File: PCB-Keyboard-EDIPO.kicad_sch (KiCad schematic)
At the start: 0 parts

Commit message: MCU Edits
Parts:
- added C1: 1u, symbol Device:C_Small
- added C2, C3: 22p, symbol Device:C_Small
- added C4, C5, C6, C7: 0.1u, symbol Device:C_Small
- added C8: 10u, symbol Device:C_Small
- added J1: AVR-ISP-6, symbol Connector:AVR-ISP-6
- added R1: 10k, symbol Device:R_Small
- added U1: ATmega32U4-A, Package_QFP:TQFP-44_10x10mm_P0.8mm, symbol MCU_Microchip_ATmega:ATmega32U4-A
- added Y1: XTAL, symbol Device:Crystal_GND24_Small
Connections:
- new net: R1.1, U1.33 (~{HWB}/PE2)
- new net: C1.1, U1.6 (UCAP)
- new net +5V: C4.1, C5.1, C6.1, C7.1, C8.1, J1.2 (VCC), U1.14 (VCC), U1.2 (UVCC), U1.24 (AVCC), U1.34 (VCC), U1.44 (AVCC)
- new net D+: U1.4 (D+)
- new net D-: U1.3 (D-)
- new net GND: C1.2, C2.2, C3.2, C4.2, C5.2, C6.2, C7.2, C8.2, J1.6 (GND), R1.2, U1.15 (GND), U1.23 (GND), U1.35 (GND), U1.43 (GND), U1.5 (UGND), Y1.2, Y1.4
- new net MISO: J1.1 (MISO), U1.11 (PB3)
- new net MOSI: J1.4 (MOSI), U1.10 (PB2)
- new net RESET: U1.13 (~{RESET})
- new net RST: J1.5 (~{RST})
- new net SCK: J1.3 (SCK), U1.9 (PB1)
- new net XTAL1: C3.1, U1.17 (XTAL1), Y1.1
- new net XTAL2: C2.1, U1.16 (XTAL2), Y1.3
- no-connect marks 0 -> 2

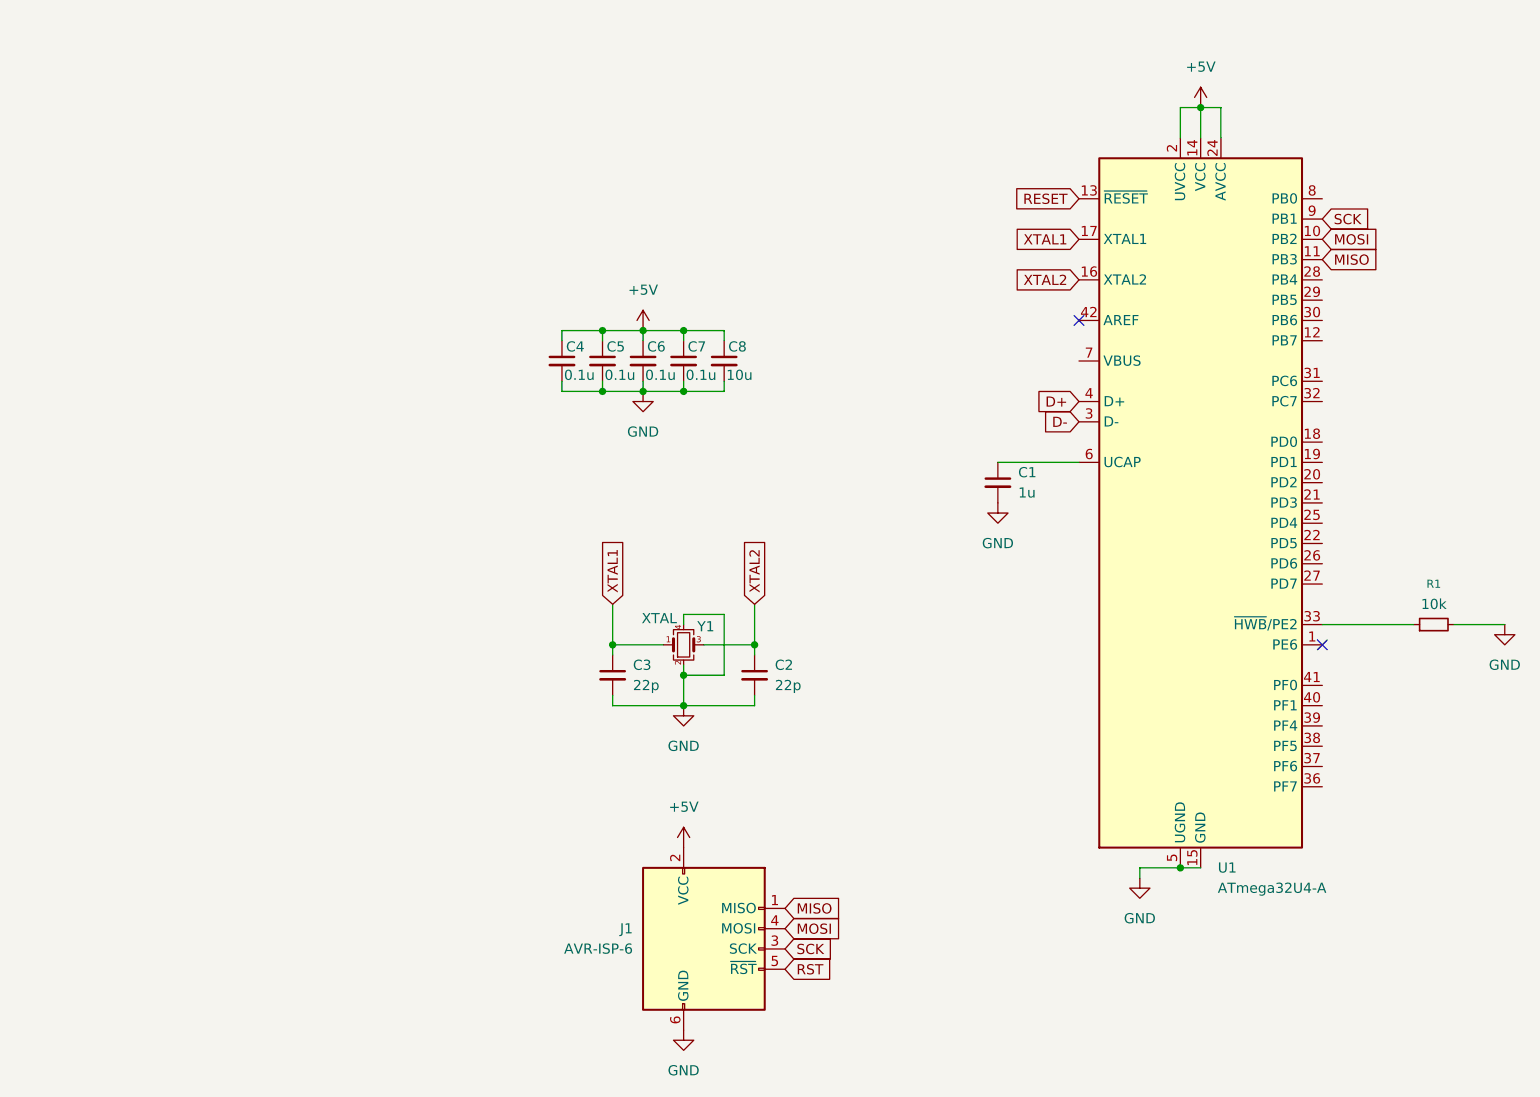
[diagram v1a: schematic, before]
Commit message: Part 1
MCU, USB Port, Switch Matrix
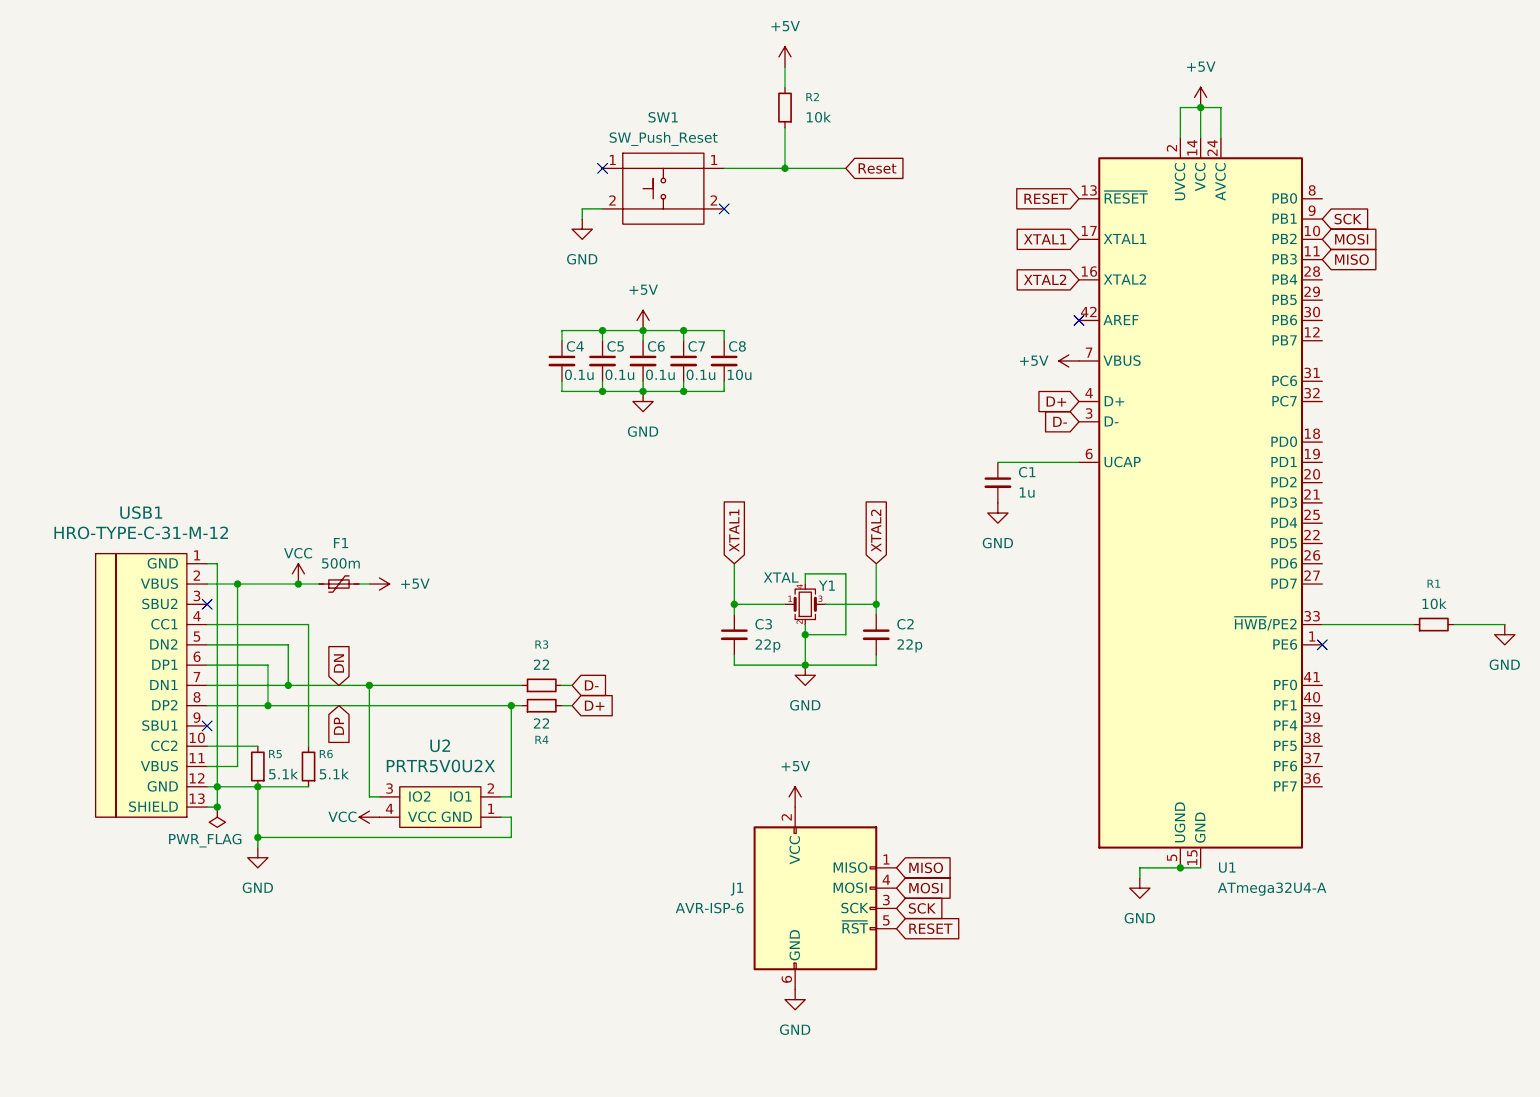
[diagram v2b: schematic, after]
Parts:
- added F1: 500m, symbol Device:Polyfuse_Small
- added R2: 10k, symbol Device:R_Small
- added R3, R4: 22, symbol Device:R_Small
- added R5, R6: 5.1k, symbol Device:R_Small
- added SW1: SW_Push_Reset, symbol local:SW_SKQG
- added U2: PRTR5V0U2X, symbol random-keyboard-parts:PRTR5V0U2X
- added USB1: HRO-TYPE-C-31-M-12, symbol Type-C:HRO-TYPE-C-31-M-12
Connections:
- net RST is gone; now on net RESET: J1.5 (~{RST})
- net +5V: now also U1.7 (VBUS), F1.2, R2.2
- net D+: now also R4.2
- net D-: now also R3.2
- net GND: now also R5.1, R6.1, SW1.2, U2.1 (GND), USB1.1 (GND), USB1.12 (GND), USB1.13 (SHIELD)
- new net: R5.2, USB1.10 (CC2)
- new net: R6.2, USB1.4 (CC1)
- new net DN: R3.1, U2.3 (IO2), USB1.5 (DN2), USB1.7 (DN1)
- new net DP: R4.1, U2.2 (IO1), USB1.6 (DP1), USB1.8 (DP2)
- new net Reset: R2.1, SW1.1
- new net VCC: F1.1, U2.4 (VCC), USB1.11 (VBUS), USB1.2 (VBUS)
- no-connect marks 2 -> 6
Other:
- moved on the sheet: C2, C3, J1, Y1
